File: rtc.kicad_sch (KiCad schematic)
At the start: 9 parts, among them IC1 DS12C887+, U2 74LS02, U37 74LS04, U47 74LS245, U50 74LS373

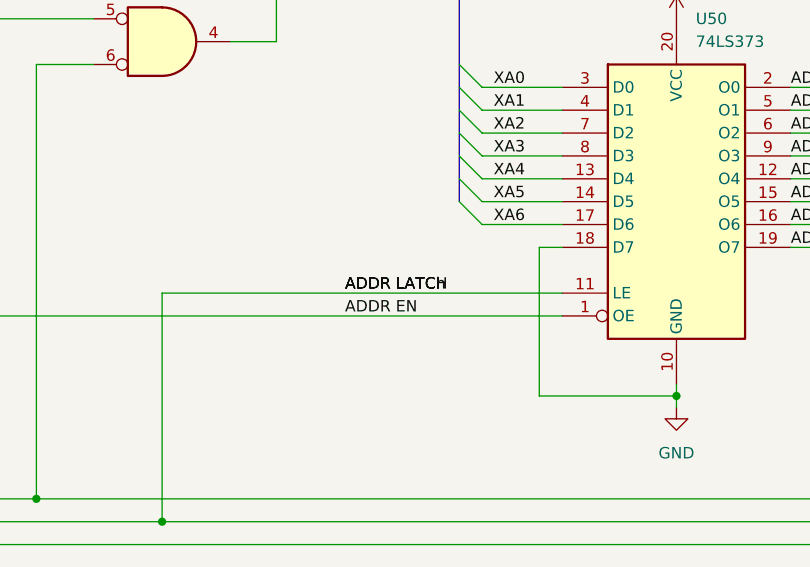
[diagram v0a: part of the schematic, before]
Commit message: fixed things
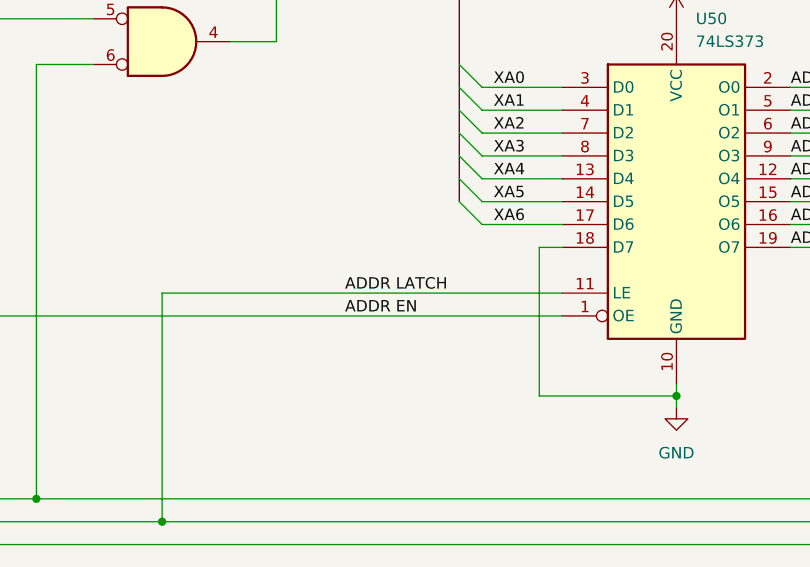
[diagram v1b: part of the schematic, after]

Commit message: Upgraded speaker, esd protection, added dip sockets, adjusted routing
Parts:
- U2, U37: footprint Package_DIP:DIP-14_W7.62mm -> Package_DIP:DIP-14_W7.62mm_Socket
- U47, U50: footprint Package_DIP:DIP-20_W7.62mm -> Package_DIP:DIP-20_W7.62mm_Socket
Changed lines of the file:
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@@
 			)
 		)
-		(property "Footprint" "Package_DIP:DIP-14_W7.62mm"
+		(property "Footprint" "Package_DIP:DIP-14_W7.62mm_Socket"
 			(at 237.49 102.87 0)
 			(hide yes)
@@
 		)
 		(property "Sim.Type" ""
+			(at 237.49 102.87 0)
+			(hide yes)
+			(show_name no)
+			(do_not_autoplace no)
+			(effects
+				(font
+					(size 1.27 1.27)
+				)
+			)
+		)
+		(property "Sim.Device" ""
 			(at 237.49 102.87 0)
 			(hide yes)
@@
 			)
 		)
+		(property "Sim.Device" ""
+			(at 274.32 25.4 0)
+			(hide yes)
+			(show_name no)
+			(do_not_autoplace no)
+			(effects
+				(font
+					(size 1.27 1.27)
+				)
+			)
+		)
 		(pin "2"
 		)
@@
 			)
 		)
+		(property "Sim.Device" ""
+			(at 186.69 105.41 0)
+			(hide yes)
+			(show_name no)
+			(do_not_autoplace no)
+			(effects
+				(font
+					(size 1.27 1.27)
+				)
+			)
+		)
 		(pin "17"
 		)
@@
 			)
 		)
-		(property "Footprint" "Package_DIP:DIP-20_W7.62mm"
+		(property "Footprint" "Package_DIP:DIP-20_W7.62mm_Socket"
 			(at 142.24 107.95 0)
 			(hide yes)
@@
 		)
 		(property "Sim.Type" ""
+			(at 142.24 107.95 0)
+			(hide yes)
+			(show_name no)
+			(do_not_autoplace no)
+			(effects
+				(font
+					(size 1.27 1.27)
+				)
+			)
+		)
+		(property "Sim.Device" ""
 			(at 142.24 107.95 0)
 			(hide yes)
@@
 			)
 		)
+		(property "Sim.Device" ""
+			(at 260.35 25.4 0)
+			(hide yes)
+			(show_name no)
+			(do_not_autoplace no)
+			(effects
+				(font
+					(size 1.27 1.27)
+				)
+			)
+		)
 		(pin "2"
 		)
@@
 			)
 		)
-		(property "Footprint" "Package_DIP:DIP-20_W7.62mm"
+		(property "Footprint" "Package_DIP:DIP-20_W7.62mm_Socket"
 			(at 142.24 49.53 0)
 			(hide yes)
@@
 		)
 		(property "Sim.Type" ""
+			(at 142.24 49.53 0)
+			(hide yes)
+			(show_name no)
+			(do_not_autoplace no)
+			(effects
+				(font
+					(size 1.27 1.27)
+				)
+			)
+		)
+		(property "Sim.Device" ""
 			(at 142.24 49.53 0)
 			(hide yes)
@@
 			)
 		)
-		(property "Footprint" "Package_DIP:DIP-14_W7.62mm"
+		(property "Footprint" "Package_DIP:DIP-14_W7.62mm_Socket"
 			(at 76.2 77.47 0)
 			(hide yes)
@@
 		)
 		(property "Sim.Type" ""
+			(at 76.2 77.47 0)
+			(hide yes)
+			(show_name no)
+			(do_not_autoplace no)
+			(effects
+				(font
+					(size 1.27 1.27)
+				)
+			)
+		)
+		(property "Sim.Device" ""
 			(at 76.2 77.47 0)
 			(hide yes)
@@
 			)
 		)
+		(property "Sim.Device" ""
+			(at 223.52 71.12 0)
+			(hide yes)
+			(show_name no)
+			(do_not_autoplace no)
+			(effects
+				(font
+					(size 1.27 1.27)
+				)
+			)
+		)
 		(pin "1"
 		)
@@
 			)
 		)
-		(property "Footprint" "Package_DIP:DIP-14_W7.62mm"
+		(property "Footprint" "Package_DIP:DIP-14_W7.62mm_Socket"
 			(at 85.09 90.17 0)
 			(hide yes)
@@
 		)
 		(property "Sim.Type" ""
+			(at 85.09 90.17 0)
+			(hide yes)
+			(show_name no)
+			(do_not_autoplace no)
+			(effects
+				(font
+					(size 1.27 1.27)
+				)
+			)
+		)
+		(property "Sim.Device" ""
 			(at 85.09 90.17 0)
 			(hide yes)
@@
 			(at 246.38 25.4 0)
 			(hide yes)
+			(show_name no)
+			(do_not_autoplace no)
+			(effects
+				(font
+					(size 1.27 1.27)
+				)
+			)
+		)
+		(property "Sim.Device" ""
+			(at 246.38 25.4 0)
+			(hide yes)
